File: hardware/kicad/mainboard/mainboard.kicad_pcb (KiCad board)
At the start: 2 copper layers, 100 x 100 mm, 50 parts, among them J1 USB-C 5V/3A (GCT USB4085), J10 Stepper 1A 1B 2A 2B, J2 IDC 2x15 -> Frontpanel, J3 Servo Pan (GND/5V/Sig), J4 Servo Tilt (GND/5V/Sig), J5 ARGB 5V/GND/Data, J6 BME680 (VCC GND SCL SDA SDO C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, J7 Augen-Kabel, J8 RST/BOOT extern, U1 ESP32-S3-DevKitC-1-N16R8, U2 LD1117V33, U3 DRV8833 Pololu #2130, U4 DRV8833 Pololu #2130 (Fader 3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, U5 MT3608 Boost ~9V (optional, 4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, U6 ESP32-C3 SuperMini Reserve, U7 A4988/TMC2209 Reserve

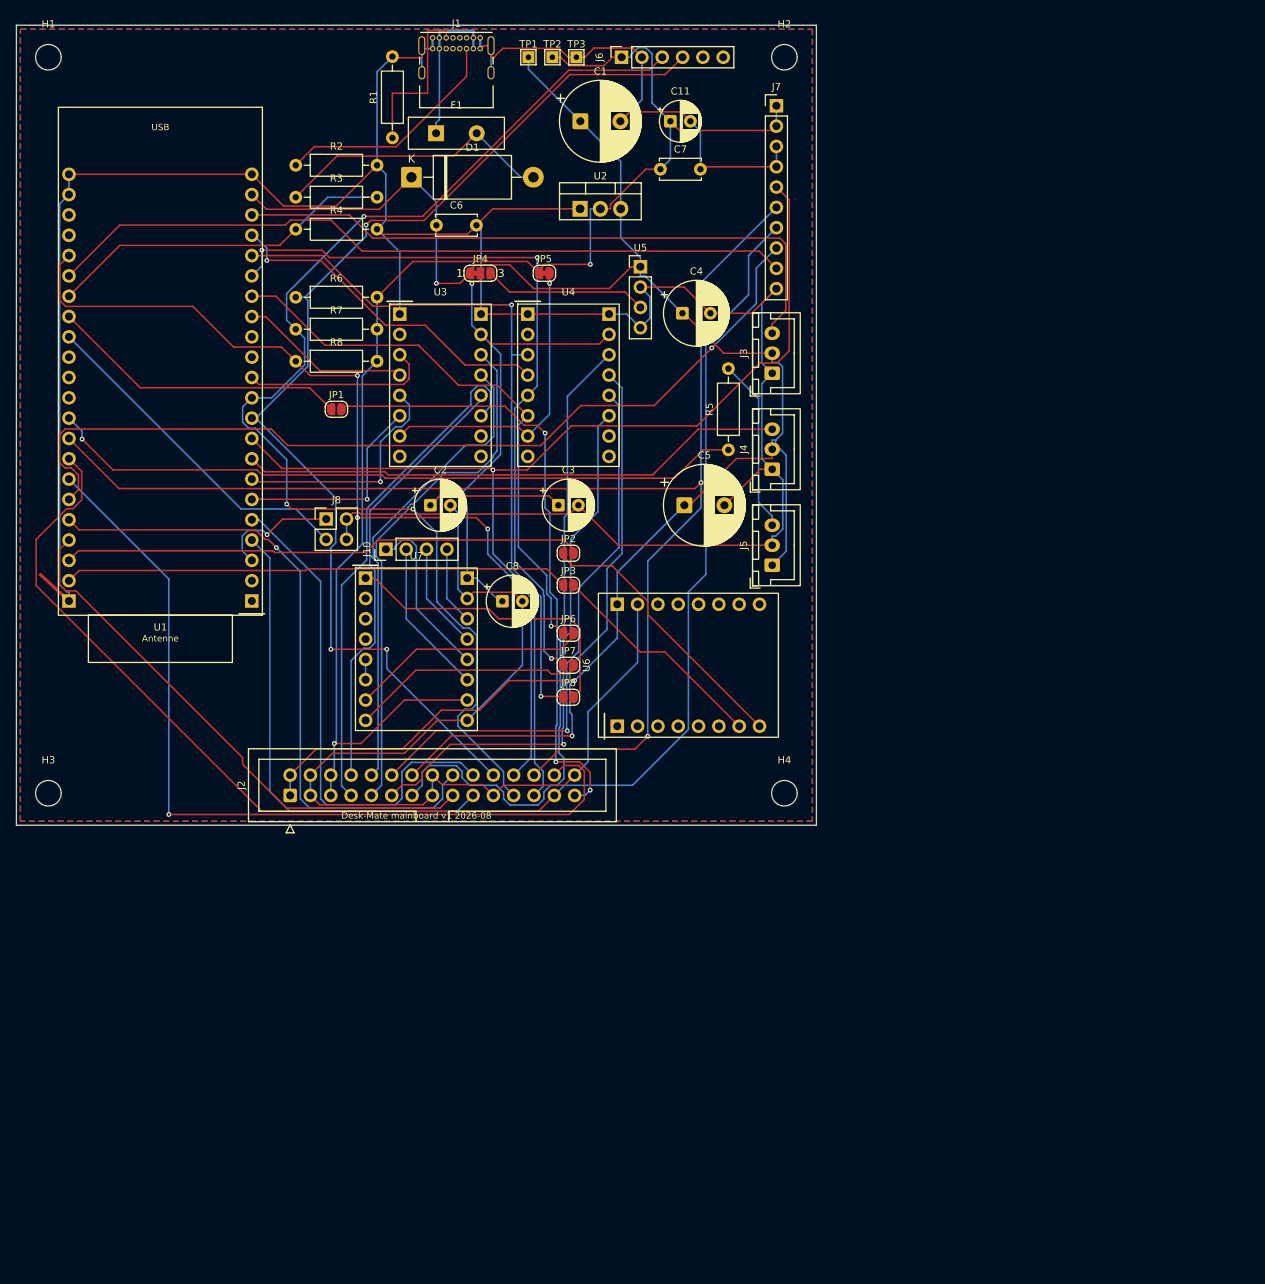
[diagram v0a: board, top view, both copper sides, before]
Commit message: Session 2026-08-31 12:22: Arbeitsstand
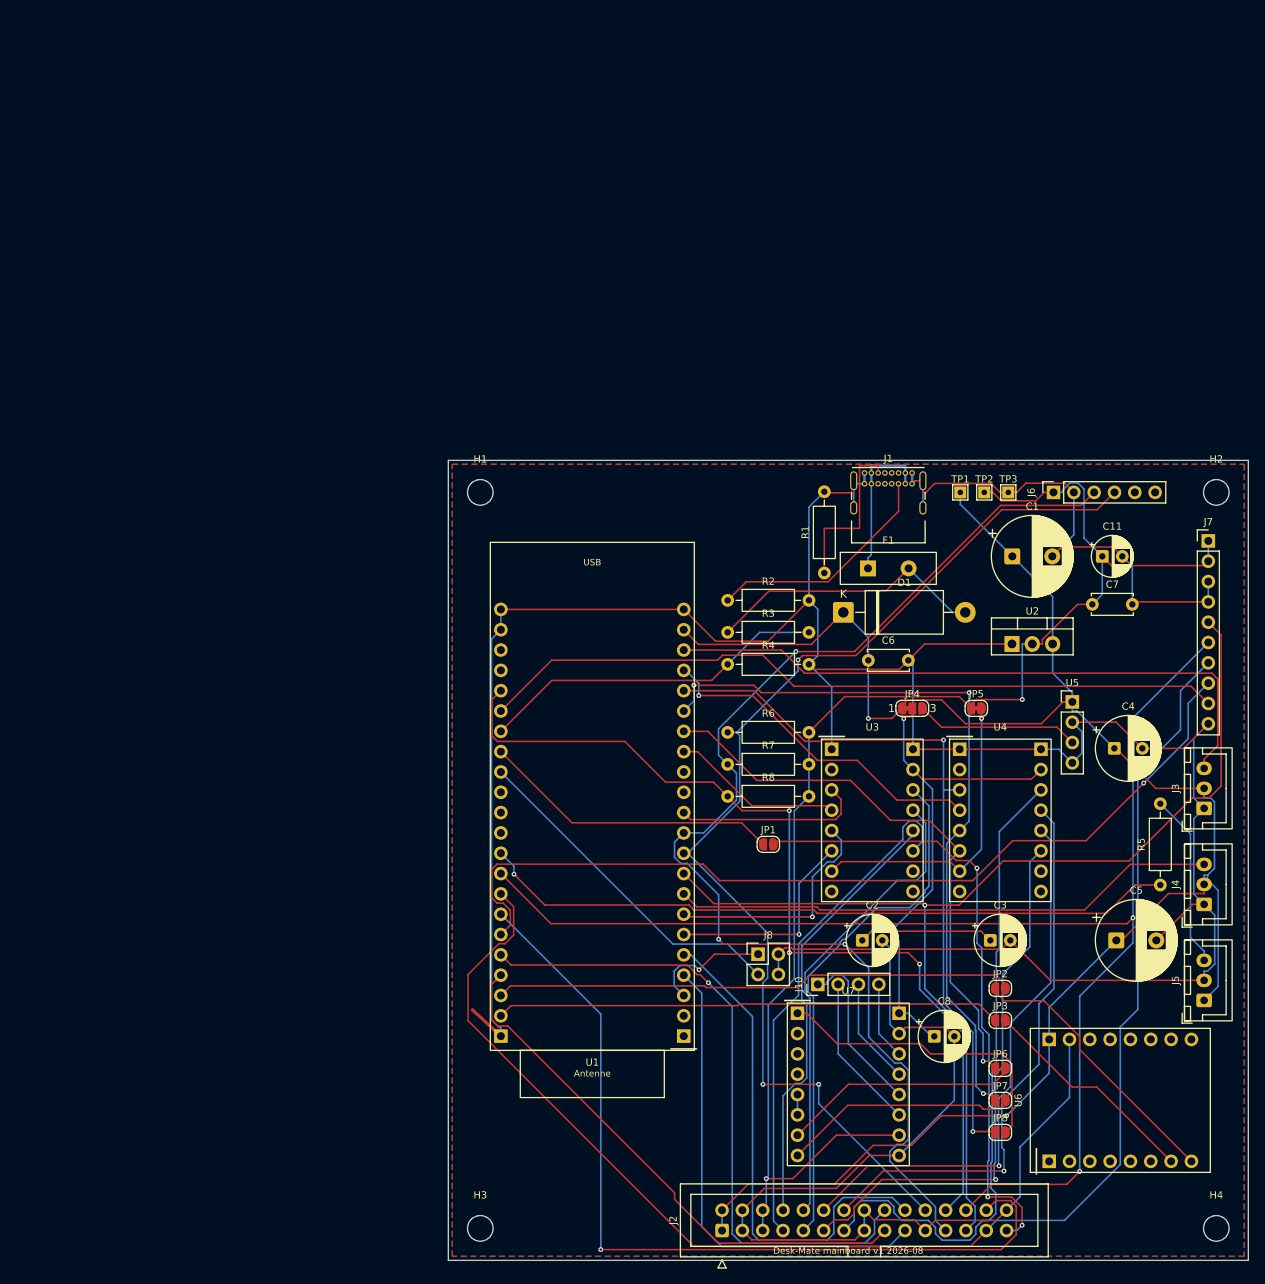
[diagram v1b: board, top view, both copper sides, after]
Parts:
- moved C7 76.6 mm to (134.5, 72.4)
- moved D1 76.6 mm to (103.4, 73.4)
- moved H1 76.6 mm to (58.0, 58.4)
- moved J1 76.6 mm to (106.0, 56.0)
- moved J10 76.6 mm to (100.2, 119.9)
- moved J3 76.6 mm to (148.5, 97.9)
- moved J4 76.6 mm to (148.5, 109.9)
- moved J5 76.6 mm to (148.5, 121.9)
- moved R5 76.6 mm to (143.0, 107.5)
- moved U2 76.6 mm to (124.5, 77.3)
- moved U5 76.6 mm to (132.0, 84.6)
- moved C1 76.6 mm to (124.5, 66.4)
- moved C11 76.6 mm to (135.7, 66.4)
- moved C2 76.6 mm to (105.7, 114.4)
- moved C3 76.6 mm to (121.7, 114.4)
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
